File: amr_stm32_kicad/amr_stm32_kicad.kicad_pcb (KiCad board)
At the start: 4 copper layers, 85 x 56 mm, 96 parts, among them J1 Header 2x20, J10 VCC, J2 Motor_Left, J3 Motor_right, J4 ST_Link, J5 USB_FS_Interface, J6 USB_UART, J7 +12V_BAT, J8 USB_A_Pi, J9 UART, Q1 FDN304P, SW1 SW_Reset, SW2 SW_BOOT, U2 SGM2205-3.3, U3 BMI323, U4 TB6612FNG, U5 STM32F405RGTx, U6 LM358, U7 CH340E, U9 TPS56528DDA, Y2 8MHz

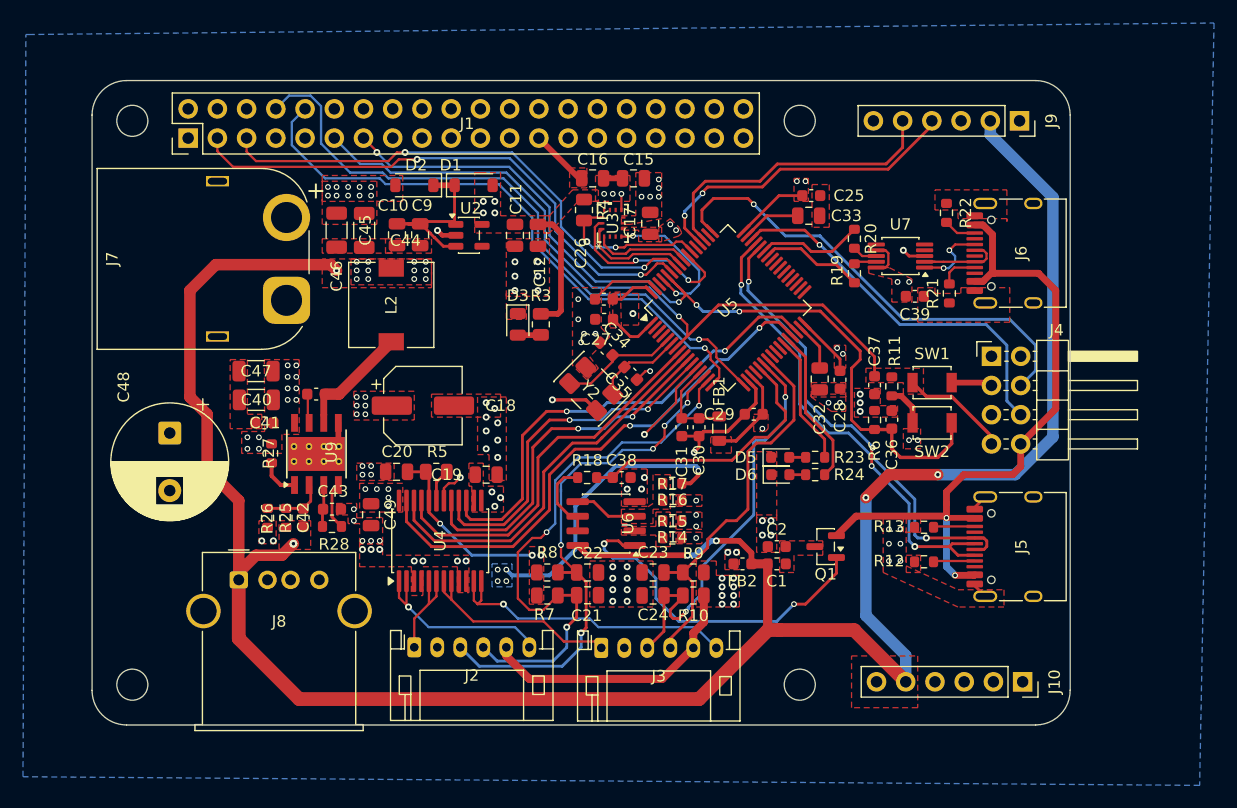
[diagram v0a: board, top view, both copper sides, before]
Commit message: update15
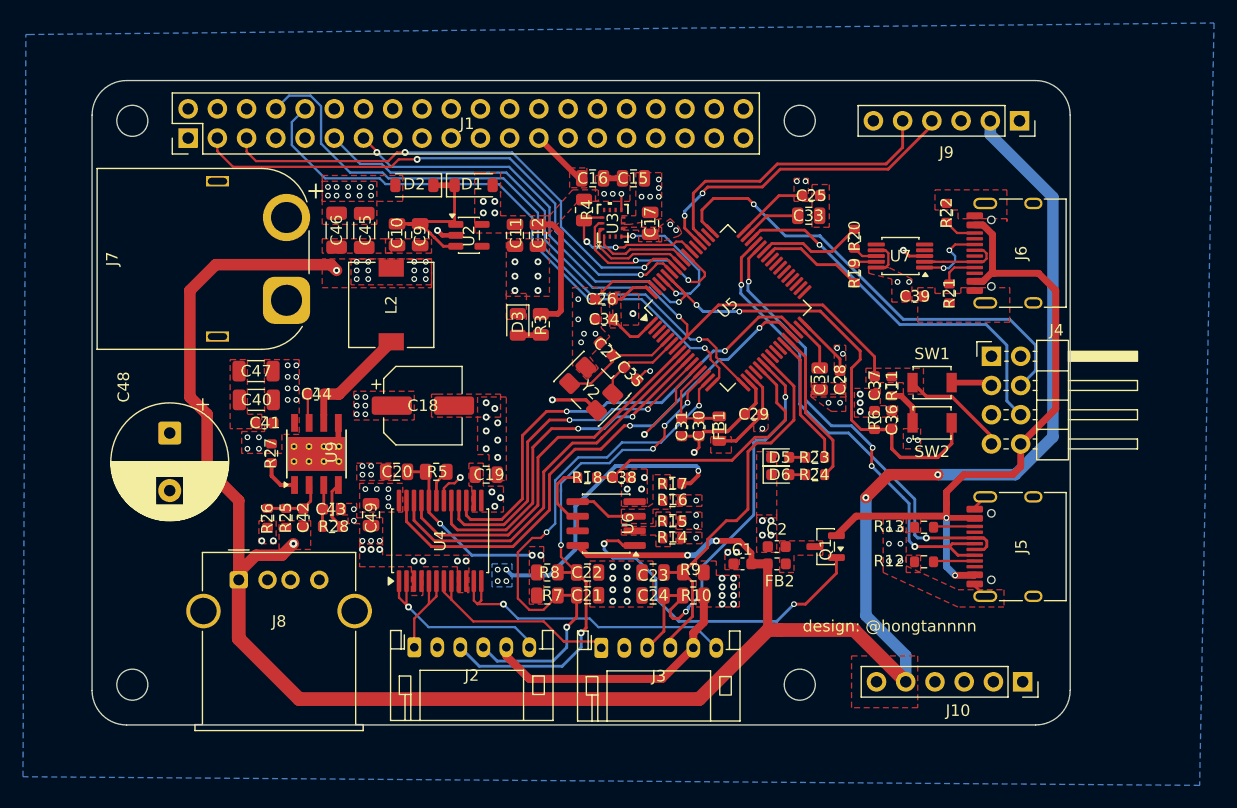
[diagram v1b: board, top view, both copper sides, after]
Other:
- board text added: "design: @hongtannnn"
